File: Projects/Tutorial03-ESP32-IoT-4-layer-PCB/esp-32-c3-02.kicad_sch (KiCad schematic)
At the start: 16 parts, among them J3 GSD090012SEU, U3 ESP32-C3-WROOM-02-H4, U4 CP2102N-Axx-xQFN20, U5 USBLC6-2SC6, U6 W25Q32JVSSIQ

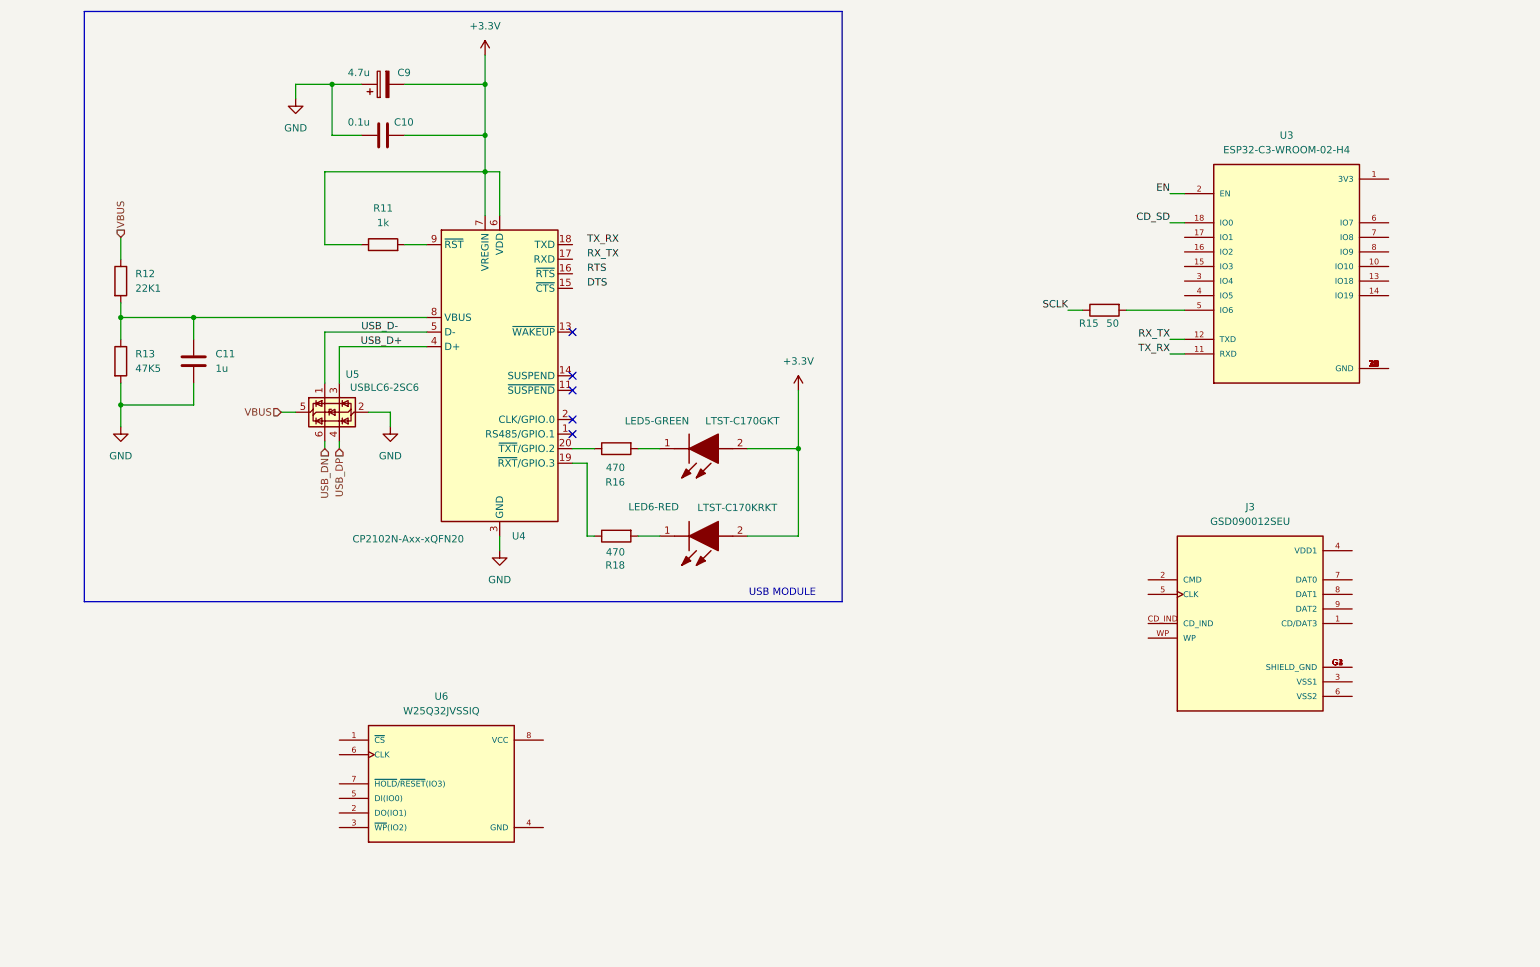
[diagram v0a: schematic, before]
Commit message: 20260308
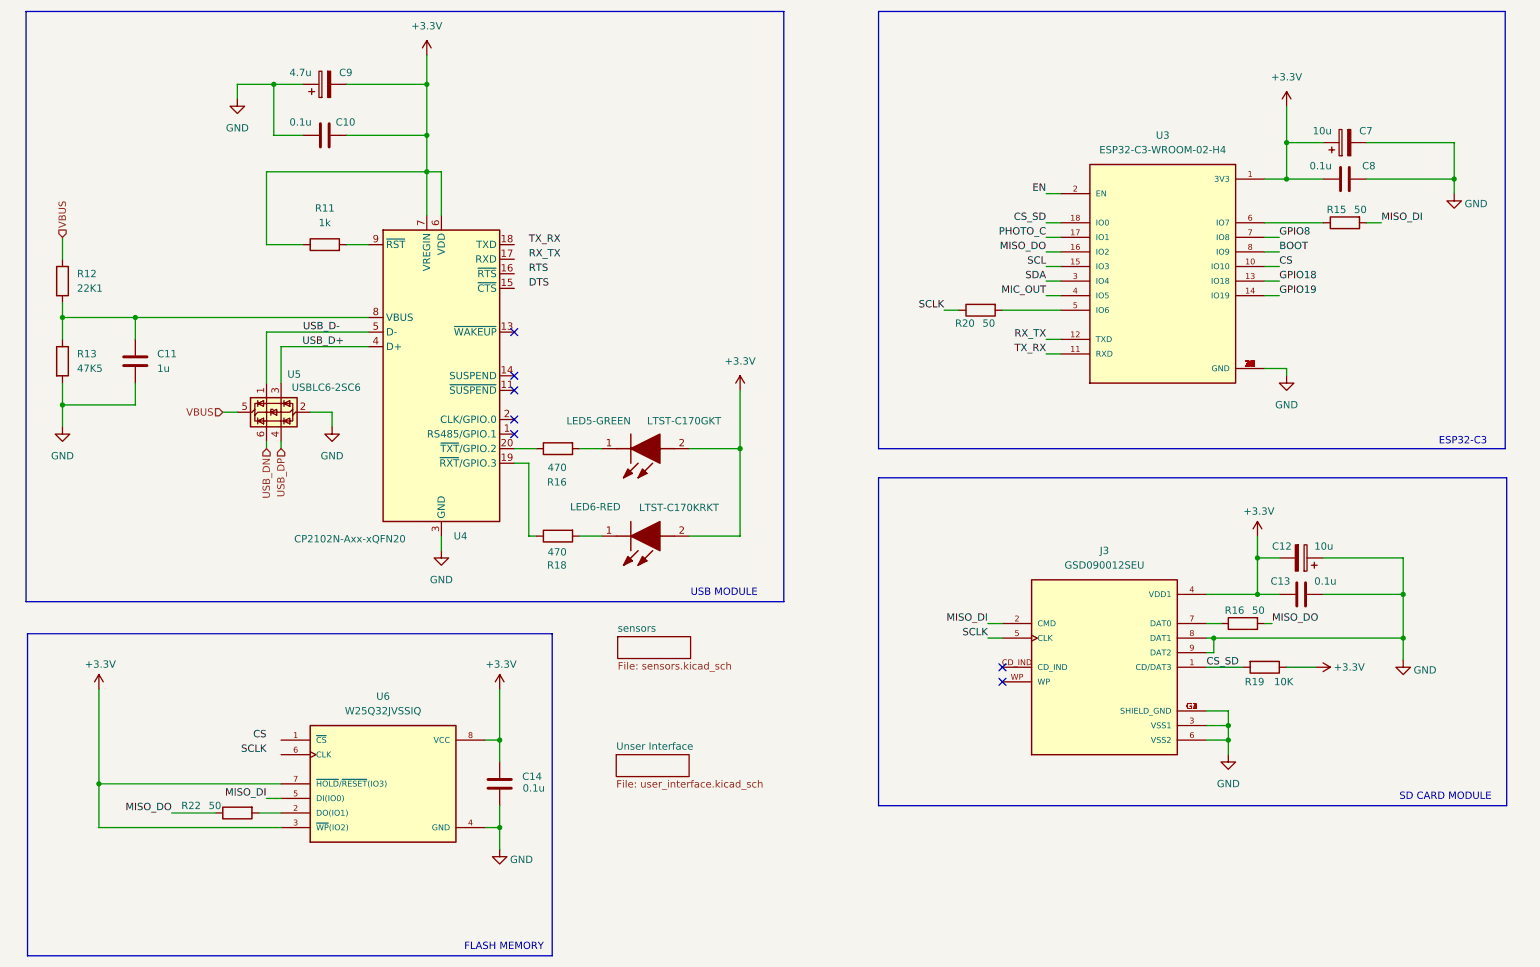
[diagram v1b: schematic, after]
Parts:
- added C12, C7: 10u, symbol Device:C_Polarized
- added C13, C14, C8: 0.1u, symbol Device:C
- added R15, R16, R22: 50, symbol Device:R
- added R19: 10K, symbol Device:R
- renumbered R15 to R20
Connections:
- net CD_SD is gone; now on net CS_SD: U3.18 (IO0)
- net +3.3V: now also J3.4 (VDD1), U3.1 (3V3), U6.3 (~{WP}(IO2)), U6.7 (~{HOLD}/~{RESET}(IO3)), U6.8 (VCC), C12.2, C13.2, C14.1, C7.1, C8.1, R19.1
- net GND: now also J3.3 (VSS1), J3.6 (VSS2), J3.8 (DAT1), J3.9 (DAT2), J3.G1 (SHIELD_GND), J3.G2 (SHIELD_GND), J3.G3 (SHIELD_GND), J3.G4 (SHIELD_GND), U3.19 (GND), U3.20 (GND), U3.21 (GND), U3.22 (GND), U3.23 (GND), U3.24 (GND), U3.25 (GND), U3.26 (GND), U3.27 (GND), U3.28 (GND), U3.29 (GND), U3.30 (GND), U3.31 (GND), U3.32 (GND), U3.33 (GND), U3.34 (GND), U3.35 (GND), U3.36 (GND), U3.37 (GND), U3.38 (GND), U3.39 (GND), U3.9 (GND), U6.4 (GND), C12.1, C13.1, C14.2, C7.2, C8.2
- net SCLK: now also J3.5 (CLK)
- net at U6.2 (DO(IO1)): now also R22.2
- net MISO_DI: now reaches U6.5 (DI(IO0))
- net MISO_DI: now also J3.2 (CMD), R15.2
- net CS: now reaches U3.10 (IO10)
- net GPIO18: now reaches U3.13 (IO18)
- net GPIO19: now reaches U3.14 (IO19)
- net SCL: now reaches U3.15 (IO3)
- net MISO_DO: now reaches U3.16 (IO2)
- net MISO_DO: now also R16.2, R22.1
- net PHOTO_C: now reaches U3.17 (IO1)
- net SDA: now reaches U3.3 (IO4)
- net MIC_OUT: now reaches U3.4 (IO5)
- net at U3.6 (IO7): now also R15.1
- net GPIO8: now reaches U3.7 (IO8)
- net BOOT: now reaches U3.8 (IO9)
- net CS_SD: now reaches J3.1 (CD/DAT3)
- net CS_SD: now also R19.2
- net at J3.7 (DAT0): now also R16.1
- no-connect marks 5 -> 7
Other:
- added sheet Unser Interface (user_interface.kicad_sch)
- added sheet sensors (sensors.kicad_sch)
- note added: "ESP32-C3"
- note added: "FLASH MEMORY"
- note added: "SD CARD MODULE"
- moved on the sheet: C10, C11, C9, J3, LED5-GREEN, LED6-RED, R11, R12, R13, R16, R18, R20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

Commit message: 20260315
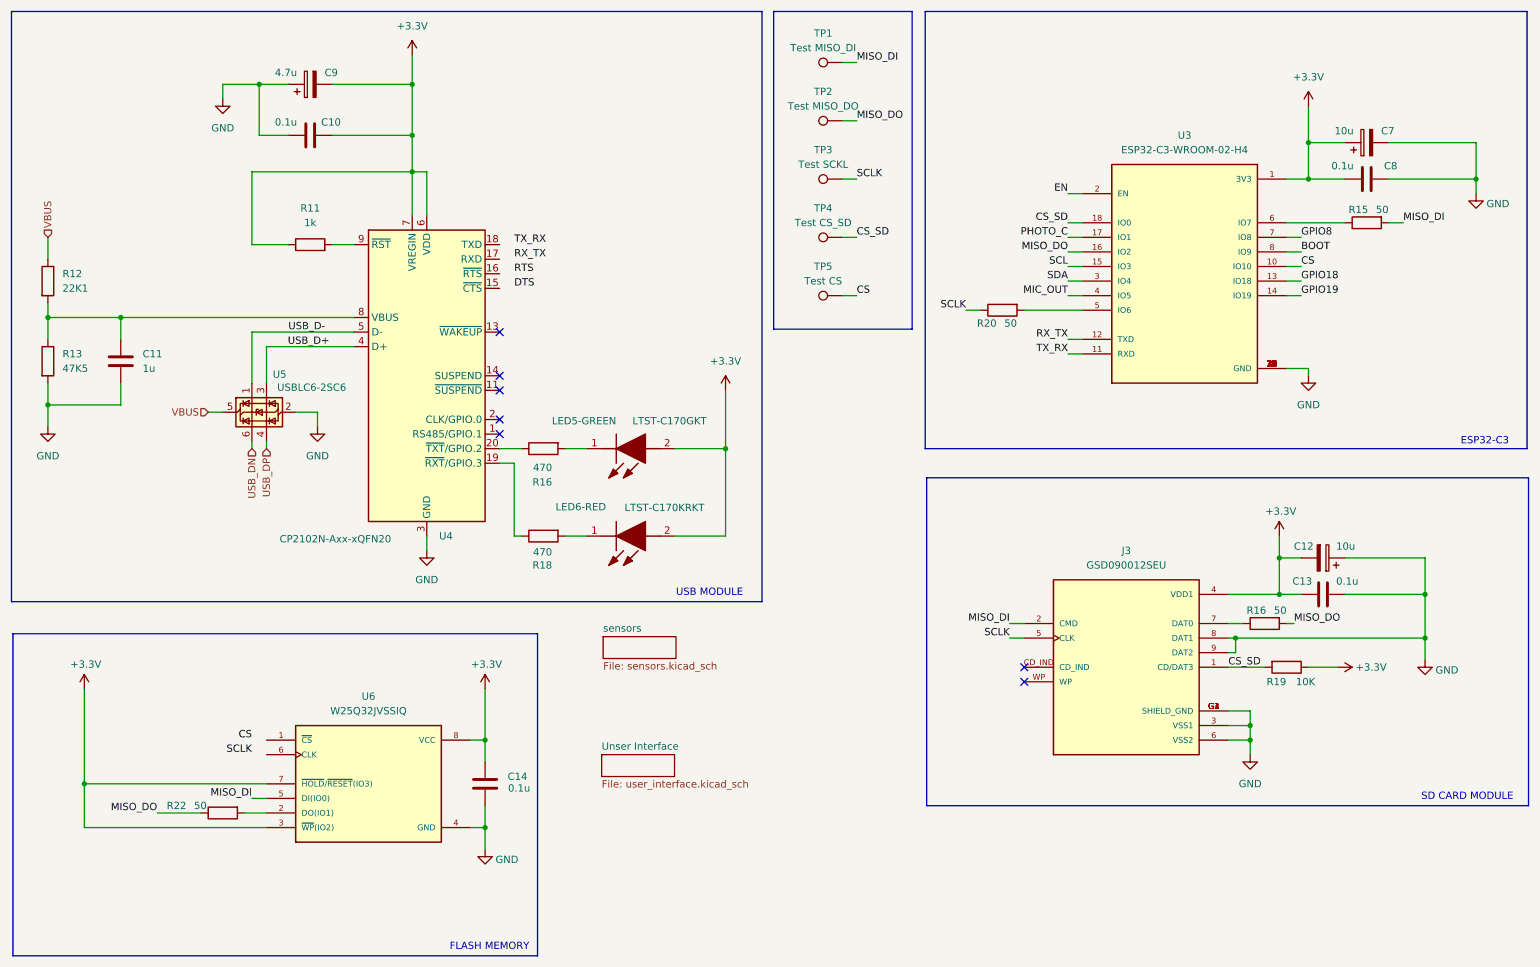
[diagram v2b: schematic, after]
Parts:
- added TP1: Test MISO_DI, symbol Connector:TestPoint
- added TP2: Test MISO_DO, symbol Connector:TestPoint
- added TP3: Test SCKL, symbol Connector:TestPoint
- added TP4: Test CS_SD, symbol Connector:TestPoint
- added TP5: Test CS, symbol Connector:TestPoint
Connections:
- net CS: now also TP5.1
- net CS_SD: now also TP4.1
- net MISO_DI: now also TP1.1
- net MISO_DO: now also TP2.1
- net SCLK: now also TP3.1
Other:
- moved on the sheet: C10, C11, C12, C13, C14, C7, C8, C9, J3, LED5-GREEN, LED6-RED, R11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

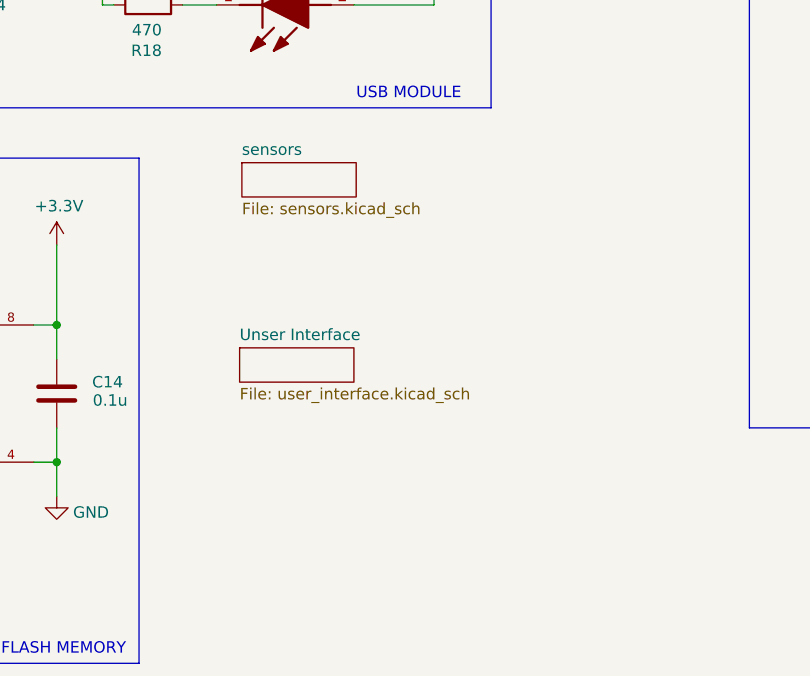
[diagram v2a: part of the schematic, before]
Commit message: 20260321
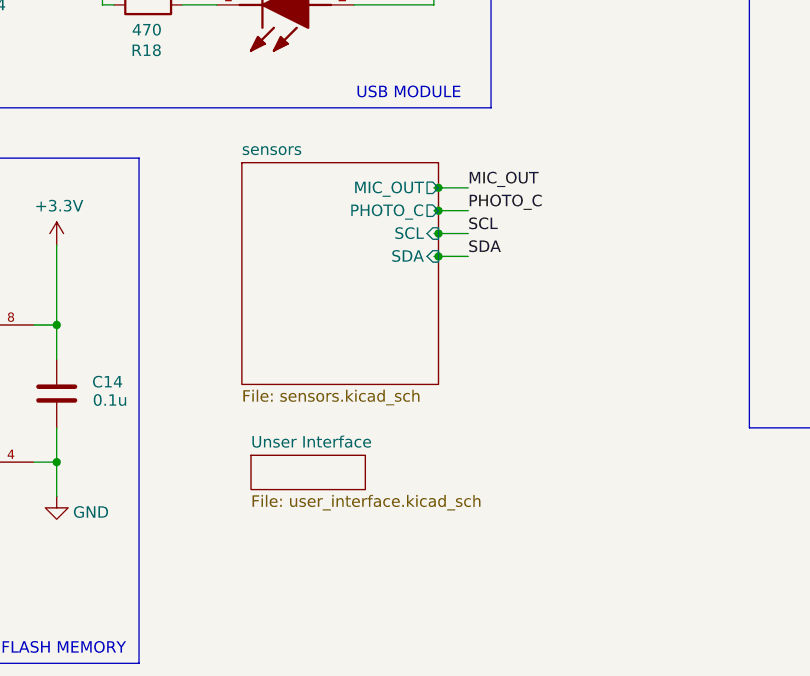
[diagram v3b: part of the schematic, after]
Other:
- sheet sensors ports: added MIC_OUT, PHOTO_C, SCL, SDA; removed none
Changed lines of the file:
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@@
 	)
 	(junction
+		(at 141.478 134.62)
+		(diameter 0)
+		(color 0 0 0 0)
+	)
+	(junction
 		(at 59.69 35.56)
 		(diameter 0)
@@
 	)
 	(junction
+		(at 141.478 142.24)
+		(diameter 0)
+		(color 0 0 0 0)
+	)
+	(junction
 		(at 271.78 52.07)
 		(diameter 0)
@@
 	)
 	(junction
+		(at 141.478 137.16)
+		(diameter 0)
+		(color 0 0 0 0)
+	)
+	(junction
 		(at 242.57 45.72)
 		(diameter 0)
@@
 		(color 0 0 0 0)
 	)
+	(junction
+		(at 141.478 139.7)
+		(diameter 0)
+		(color 0 0 0 0)
+	)
 	(no_connect
 		(at 101.6 78.74)
@@
 	(wire
 		(pts
+			(xy 140.97 137.16) (xy 141.478 137.16)
+		)
+		(stroke
+			(width 0)
+			(type default)
+		)
+	)
+	(wire
+		(pts
 			(xy 22.86 76.2) (xy 35.56 76.2)
 		)
@@
 	(wire
 		(pts
+			(xy 141.478 139.7) (xy 144.78 139.7)
+		)
+		(stroke
+			(width 0)
+			(type default)
+		)
+	)
+	(wire
+		(pts
 			(xy 99.06 149.86) (xy 99.06 153.67)
 		)
@@
 	(wire
 		(pts
+			(xy 141.478 142.24) (xy 144.78 142.24)
+		)
+		(stroke
+			(width 0)
+			(type default)
+		)
+	)
+	(wire
+		(pts
 			(xy 256.54 59.69) (xy 259.08 59.69)
 		)
@@
 	(wire
 		(pts
+			(xy 140.97 134.62) (xy 141.478 134.62)
+		)
+		(stroke
+			(width 0)
+			(type default)
+		)
+	)
+	(wire
+		(pts
 			(xy 228.6 149.86) (xy 232.41 149.86)
 		)
@@
 	(wire
 		(pts
+			(xy 141.478 134.62) (xy 144.78 134.62)
+		)
+		(stroke
+			(width 0)
+			(type default)
+		)
+	)
+	(wire
+		(pts
 			(xy 22.86 91.44) (xy 22.86 95.25)
 		)
@@
 	(wire
 		(pts
+			(xy 140.97 139.7) (xy 141.478 139.7)
+		)
+		(stroke
+			(width 0)
+			(type default)
+		)
+	)
+	(wire
+		(pts
 			(xy 99.06 161.29) (xy 99.06 165.1)
 		)
@@
 	(wire
 		(pts
+			(xy 140.97 142.24) (xy 141.478 142.24)
+		)
+		(stroke
+			(width 0)
+			(type default)
+		)
+	)
+	(wire
+		(pts
 			(xy 99.06 165.1) (xy 99.06 168.91)
 		)
@@
 	(wire
 		(pts
+			(xy 141.478 137.16) (xy 144.78 137.16)
+		)
+		(stroke
+			(width 0)
+			(type default)
+		)
+	)
+	(wire
+		(pts
 			(xy 237.49 118.11) (xy 237.49 124.46)
 		)
@@
 		)
 	)
+	(label "SCL"
+		(at 144.78 139.7 0)
+		(effects
+			(font
+				(size 1.27 1.27)
+			)
+			(justify left bottom)
+		)
+	)
 	(label "GPIO19"
 		(at 241.3 72.39 0)
@@
 		)
 	)
+	(label "SDA"
+		(at 144.78 142.24 0)
+		(effects
+			(font
+				(size 1.27 1.27)
+			)
+			(justify left bottom)
+		)
+	)
 	(label "CS"
 		(at 58.42 149.86 180)
@@
 		)
 	)
+	(label "MIC_OUT"
+		(at 144.78 134.62 0)
+		(effects
+			(font
+				(size 1.27 1.27)
+			)
+			(justify left bottom)
+		)
+	)
 	(label "MISO_DO"
 		(at 163.83 41.91 0)
@@
 		)
 	)
+	(label "PHOTO_C"
+		(at 144.78 137.16 0)
+		(effects
+			(font
+				(size 1.27 1.27)
+			)
+			(justify left bottom)
+		)
+	)
 	(label "MISO_DO"
 		(at 41.91 162.56 180)
@@
 	)
 	(sheet
-		(at 119.38 152.4)
+		(at 120.65 164.338)
 		(size 12.7 3.81)
 		(exclude_from_sim no)
@@
 		)
 		(property "Sheetname" "Unser Interface"
-			(at 119.38 151.6884 0)
+			(at 120.65 163.6264 0)
 			(effects
 				(font
@@
 		)
 		(property "Sheetfile" "user_interface.kicad_sch"
-			(at 119.38 156.7946 0)
+			(at 120.65 168.7326 0)
 			(effects
 				(font
@@
 	(sheet
 		(at 119.634 131.826)
-		(size 12.7 3.81)
+		(size 21.844 24.638)
 		(exclude_from_sim no)
 		(in_bom yes)
@@
 		)
 		(property "Sheetfile" "sensors.kicad_sch"
-			(at 119.634 136.2206 0)
+			(at 119.634 157.0486 0)
 			(effects
 				(font
@@
 			)
 		)
+		(pin "MIC_OUT" output
+			(at 141.478 134.62 0)
+			(effects
+				(font
+					(size 1.27 1.27)
+				)
+				(justify right)
+			)
+		)
+		(pin "PHOTO_C" output
+			(at 141.478 137.16 0)
+			(effects
+				(font
+					(size 1.27 1.27)
+				)
+				(justify right)
+			)
+		)
+		(pin "SCL" input
+			(at 141.478 139.7 0)
+			(effects
+				(font
+					(size 1.27 1.27)
+				)
+				(justify right)
+			)
+		)
+		(pin "SDA" input
+			(at 141.478 142.24 0)
+			(effects
+				(font
+					(size 1.27 1.27)
+				)
+				(justify right)
+			)
+		)
